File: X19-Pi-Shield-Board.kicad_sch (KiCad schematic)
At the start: 0 parts

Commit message: test
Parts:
- added C1, C2: 1uF, Package_SO:SOIC-8_3.9x4.9mm_P1.27mm, symbol Device:C
- added C3: 20pF, symbol Device:C
- added IC1: STM32C542CCT6, QFP50P900X900X160-48N, symbol STM32C542CCT6:STM32C542CCT6
- added U1: MIC5504-3.3YM5, Package_TO_SOT_SMD:SOT-23-5, symbol Regulator_Linear:MIC5504-3.3YM5
- added U2: BME280, Package_LGA:Bosch_LGA-8_2.5x2.5mm_P0.65mm_ClockwisePinNumbering, symbol Sensor:BME280
- added U3: INA237AIDGSR, VSSOP_IDGSR_TEX, symbol INA237AIDGSR:INA237AIDGSR
- added U4: TCAN1044VDRQ1, D0008A-IPC_A, symbol TCAN1044VDRQ1:TCAN1044VDRQ1
- added U5: MCP2518FDT-E/QBB, VDFN14_QBB_MCH, symbol MCP2518FDT_E_QBB:MCP2518FDT-E_QBB
- added Y1: ECS-120-18-33-JGN-TR, ECS-120-18-33-JGN-TR:XTAL_ECS-120-18-33-JGN-TR, symbol ECS-120-18-33-JGN-TR:ECS-120-18-33-JGN-TR
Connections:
- new net +3.3V: C2.1, C3.1, U1.5 (VOUT), Y1.1 (IN/OUT)
- new net +5V: C1.1, U1.1 (VIN)
- new net GND: C1.2, C2.2, C3.2, U1.2 (GND), Y1.2 (GND), Y1.3 (OUT/IN), Y1.4 (GND__1)
- new net MISO: IC1.27 (PB14)
- new net MOSI: IC1.28 (PB15)
- new net NRST: IC1.7 (NRST)

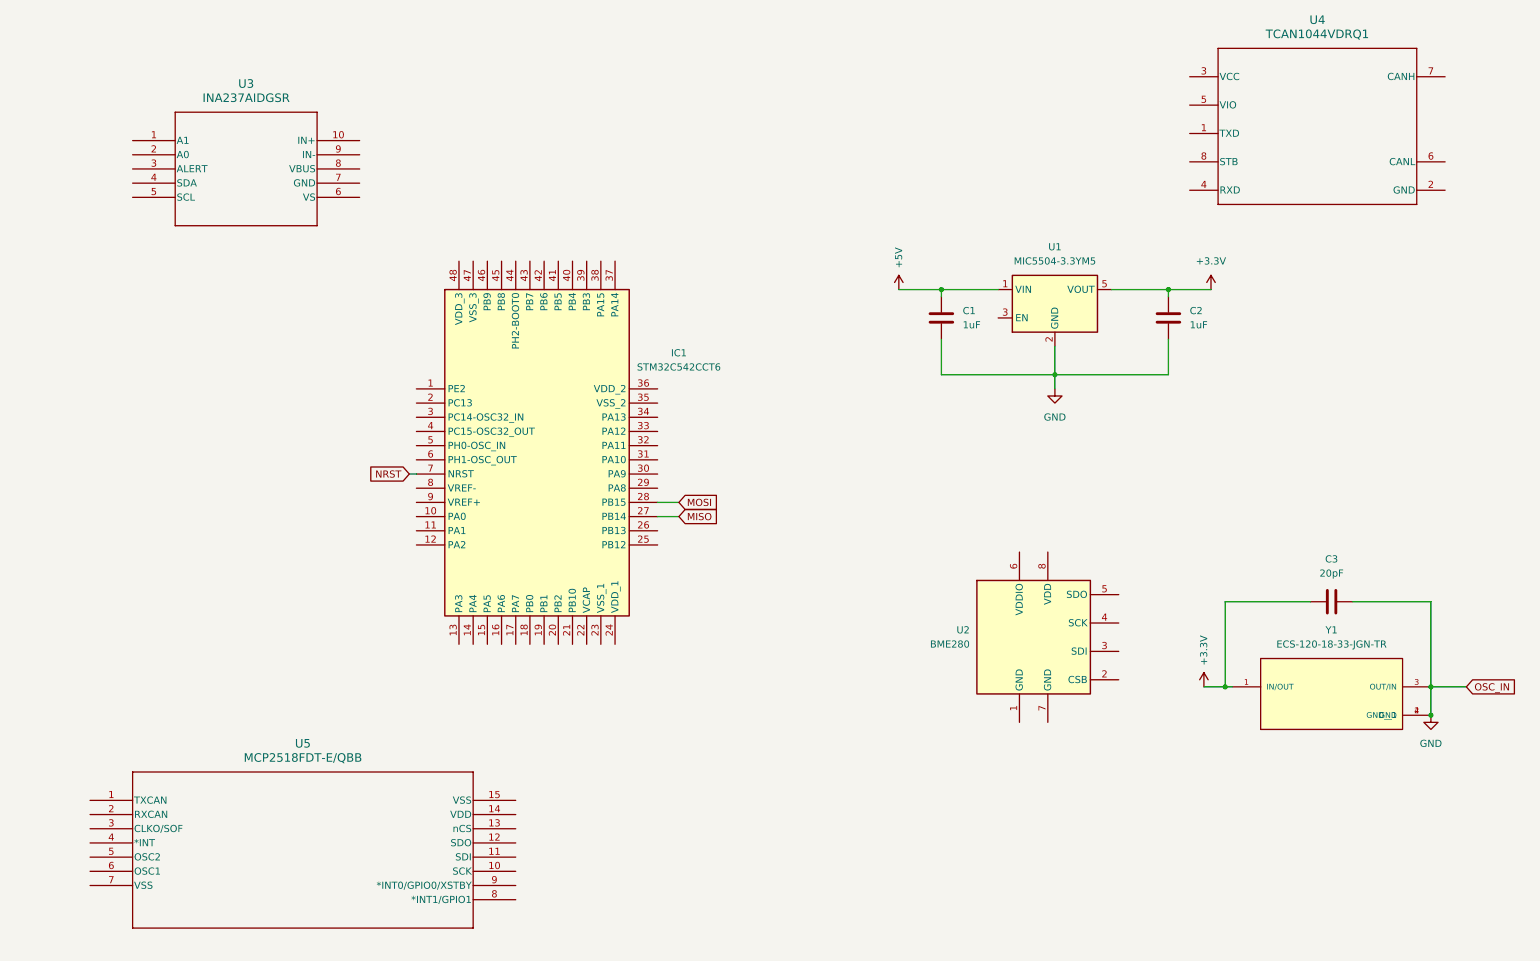
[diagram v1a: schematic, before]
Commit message: finishing board stuff
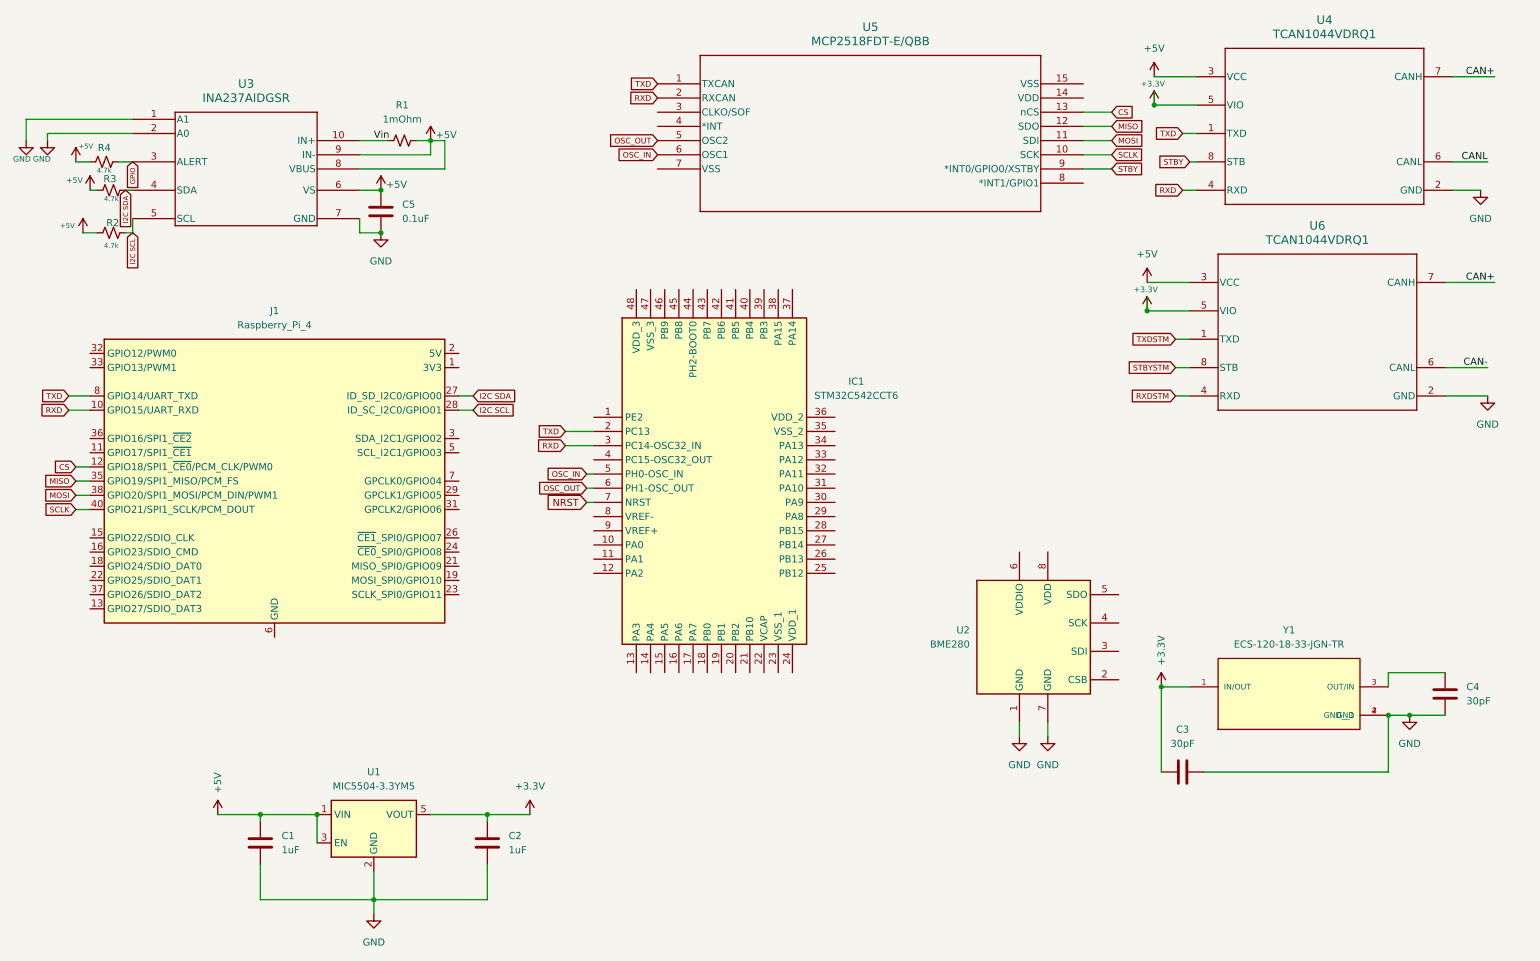
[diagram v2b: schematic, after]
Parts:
- added C4: 30pF, symbol Device:C
- added C5: 0.1uF, symbol Device:C
- added J1: Raspberry_Pi_4, symbol Connector:Raspberry_Pi_4
- added R1: 1mOhm, D0008A-IPC_A, symbol Device:R_Small_US
- added R2, R3, R4: 4.7k, symbol Device:R_Small_US
- added U6: TCAN1044VDRQ1, D0008A-IPC_A, symbol TCAN1044VDRQ1:TCAN1044VDRQ1
- C3: value 20pF -> 30pF
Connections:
- net +3.3V: now also U4.5 (VIO), U6.5 (VIO)
- net +5V: now also U1.3 (EN), U3.6 (VS), U3.8 (VBUS), U3.9 (IN-), U4.3 (VCC), C5.1, R1.2, R2.1, R3.1, R4.1, U6.3 (VCC)
- net GND: now also U2.1 (GND), U2.7 (GND), U3.1 (A1), U3.2 (A0), U3.7 (GND), U4.2 (GND), C4.2, C5.2, U6.2 (GND); no longer Y1.3 (OUT/IN)
- net MISO: now also U5.12 (SDO), J1.35 (GPIO19/SPI1_MISO/PCM_FS); no longer IC1.27 (PB14)
- net MOSI: now also U5.11 (SDI), J1.38 (GPIO20/SPI1_MOSI/PCM_DIN/PWM1); no longer IC1.28 (PB15)
- net TXD: now reaches IC1.2 (PC13)
- net TXD: now also U4.1 (TXD), U5.1 (TXCAN), J1.8 (GPIO14/UART_TXD)
- net RXD: now reaches IC1.3 (PC14-OSC32_IN)
- net RXD: now also U4.4 (RXD), U5.2 (RXCAN), J1.10 (GPIO15/UART_RXD)
- net OSC_IN: now reaches IC1.5 (PH0-OSC_IN)
- net OSC_IN: now also U5.6 (OSC1)
- net OSC_OUT: now reaches IC1.6 (PH1-OSC_OUT)
- net OSC_OUT: now also U5.5 (OSC2)
- net Vin: now reaches U3.10 (IN+)
- net Vin: now also R1.1
- net GPIO: now reaches U3.3 (ALERT)
- net GPIO: now also R4.2
- net I2C SDA: now reaches U3.4 (SDA)
- net I2C SDA: now also J1.27 (ID_SD_I2C0/GPIO00), R3.2
- net I2C SCL: now reaches U3.5 (SCL)
- net I2C SCL: now also J1.28 (ID_SC_I2C0/GPIO01), R2.2
- net SCLK: now reaches U5.10 (SCK)
- net SCLK: now also J1.40 (GPIO21/SPI1_SCLK/PCM_DOUT)
- net CS: now reaches U5.13 (nCS)
- net CS: now also J1.12 (GPIO18/SPI1_~{CE0}/PCM_CLK/PWM0)
- net STBY: now reaches U5.9 (*INT0/GPIO0/XSTBY)
- net STBY: now also U4.8 (STB)
- net CANL: now reaches U4.6 (CANL)
- net CAN+: now reaches U4.7 (CANH)
- net CAN+: now also U6.7 (CANH)
- new net: C4.1, Y1.3 (OUT/IN)
- new net: J1.1 (3V3), J1.17 (3V3)
- new net: J1.14 (GND), J1.20 (GND), J1.25 (GND), J1.30 (GND), J1.34 (GND), J1.39 (GND), J1.6 (GND), J1.9 (GND)
- new net: J1.2 (5V), J1.4 (5V)
- new net CAN-: U6.6 (CANL)
- new net RXDSTM: U6.4 (RXD)
- new net STBYSTM: U6.8 (STB)
- new net TXDSTM: U6.1 (TXD)
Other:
- moved on the sheet: C1, C2, C3, IC1, U1, U4, U5, Y1
